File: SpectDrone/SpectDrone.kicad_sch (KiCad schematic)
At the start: 76 parts, among them J1 Camera, J2 GPS, J3 Barrel_Jack, J4 BME280, J5-1 BNO055-1, J5-2 BNO055-2, Q1 FDN340P, Q2 FDN340P, SW0 SW_Push, SW1 SW_Push, SW10 SW_Push, SW2 SW_Push, SW3 SW_Push, SW4 SW_Push, SW5 SW_Push, SW6 SW_Push, SW7 SW_Push, SW8 SW_Push, SW9 SW_Push, U1 C12666MA, U2 C12666MA, U3 LM7805_TO220, U4 MCP112-300E/TO, U5 MCP112-300E/TO, U6 LM7805_TO220, U7 Teensy3.2

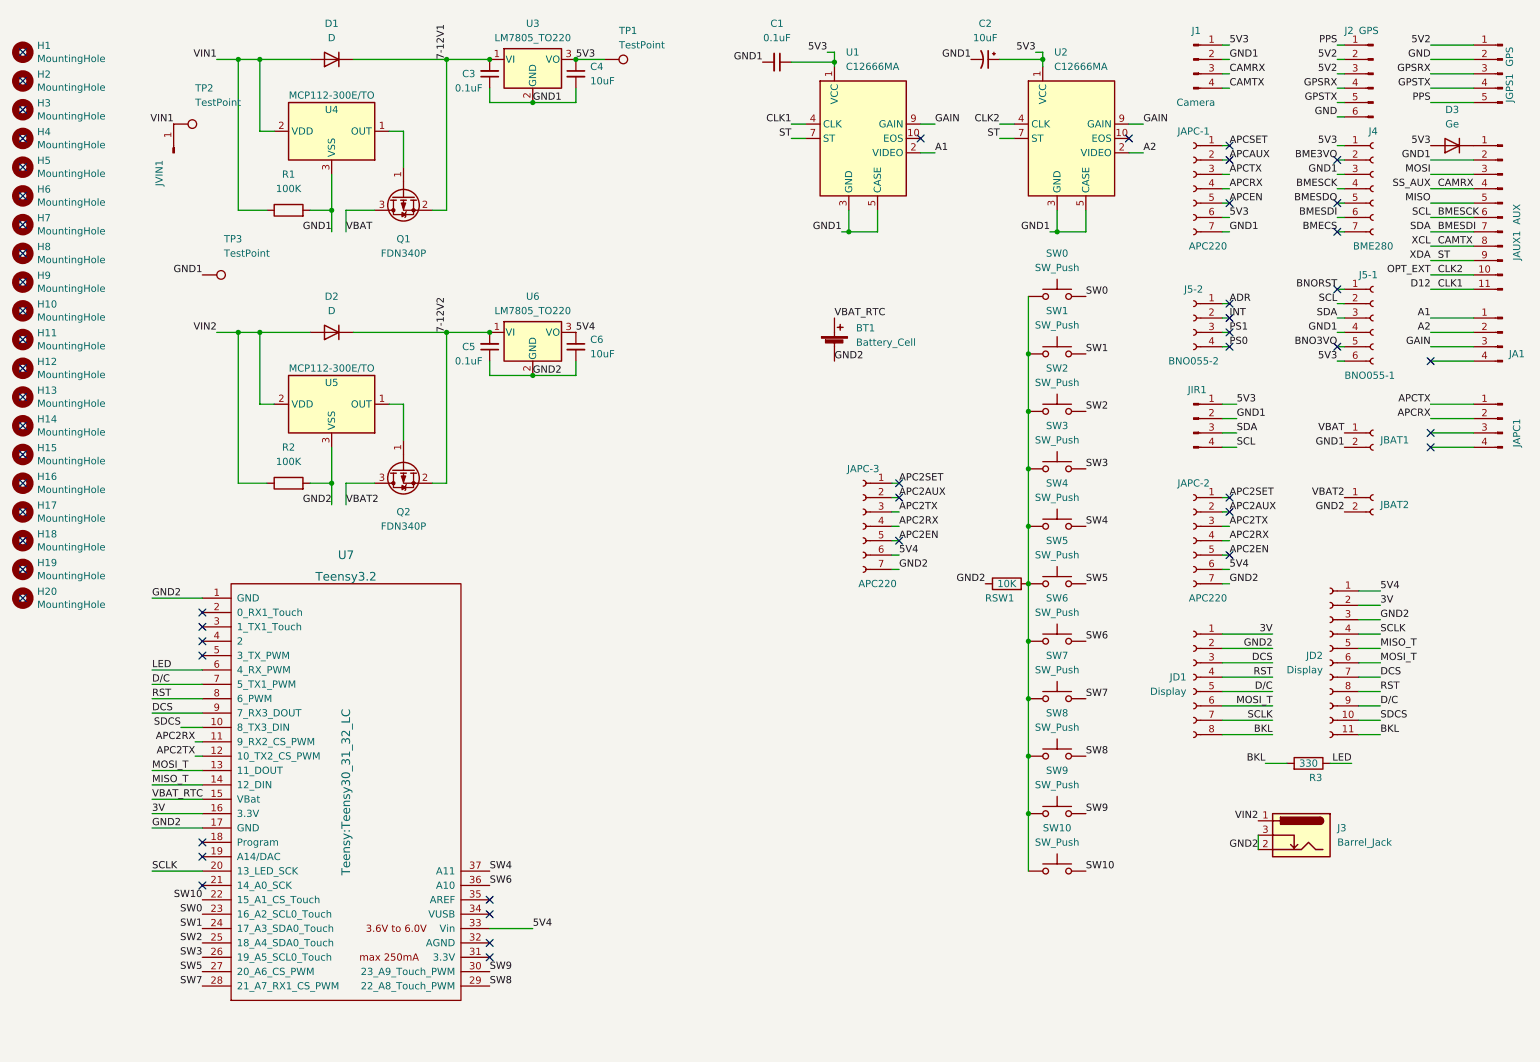
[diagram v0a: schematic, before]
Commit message: SpectDrone Development
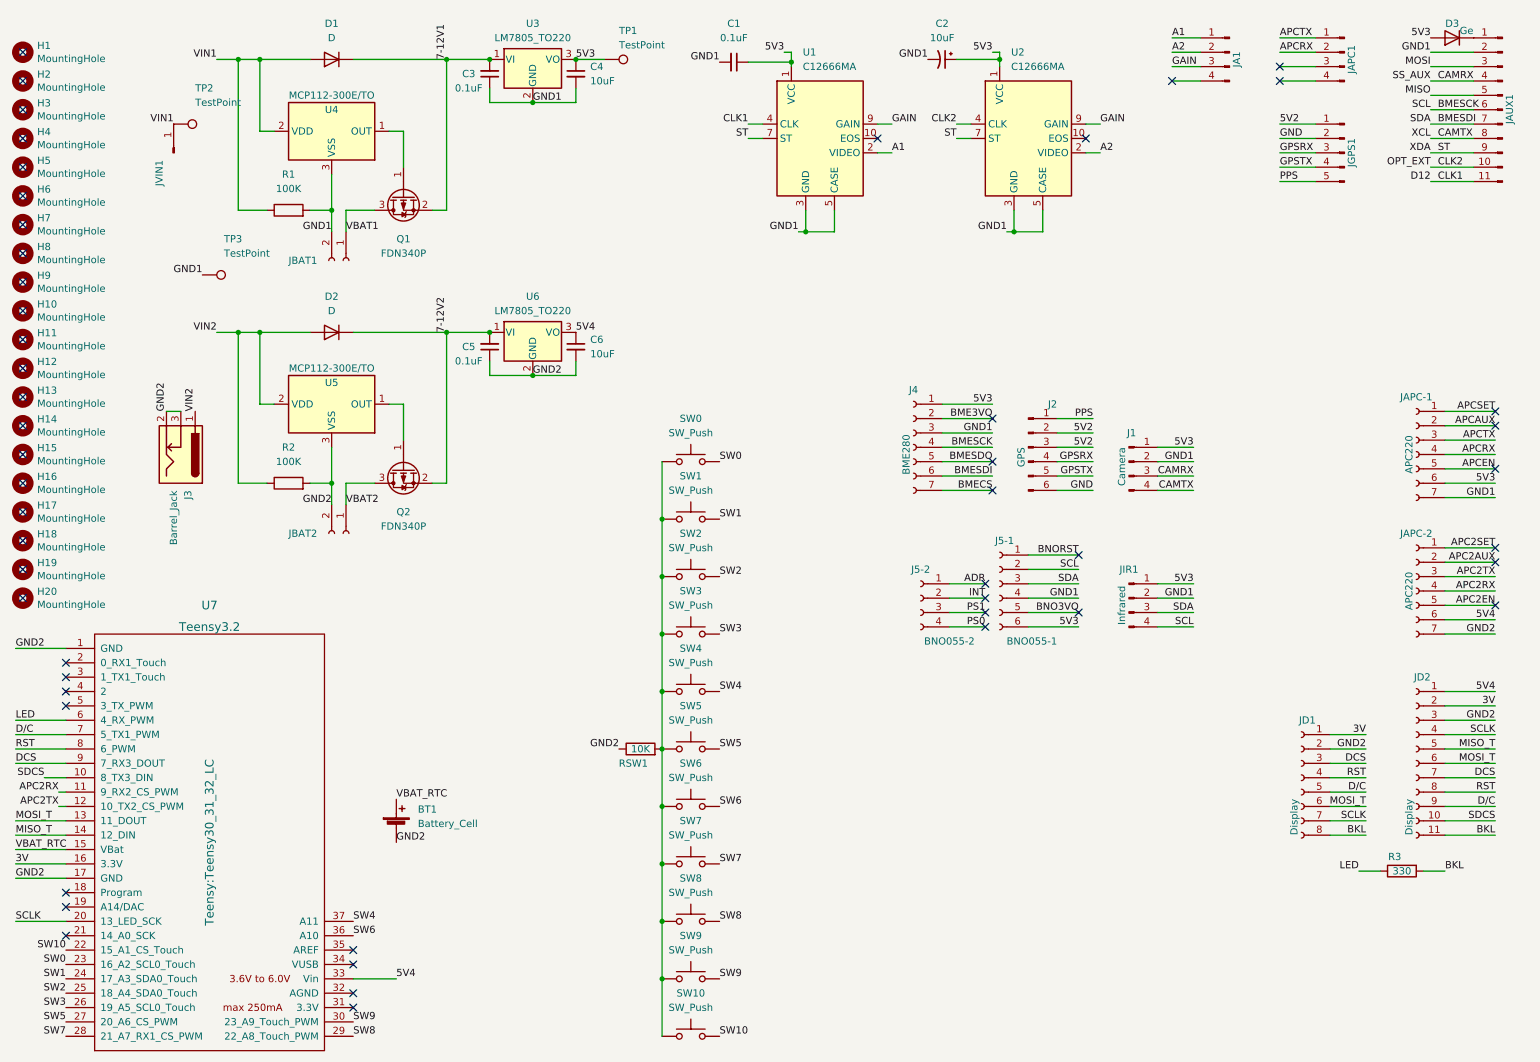
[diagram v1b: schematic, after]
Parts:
- removed JAPC-3: APC220, Connector_PinSocket_2.54mm:PinSocket_1x07_P2.54mm_Vertical, symbol Connector:Conn_01x07_Female
- JIR1: value Conn_01x04_Male -> Infrared
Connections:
- net VBAT renamed VBAT1
- no-connect marks 54 -> 51
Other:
- moved on the sheet: BT1, C1, C2, D3, J1, J2, J3, J4, J5-1, J5-2, JA1, JAPC-1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
